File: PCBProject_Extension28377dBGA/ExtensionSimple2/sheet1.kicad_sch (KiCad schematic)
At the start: 86 parts, among them P1 Header 6X2, P2 Header 6X2, P3 Header 2X2, P4 Header 2X2, P5 Header 2X2, P6 Header 2X2, Q1 FMMT618TA, U1 SN74ABT541, U2 SN74ABT541

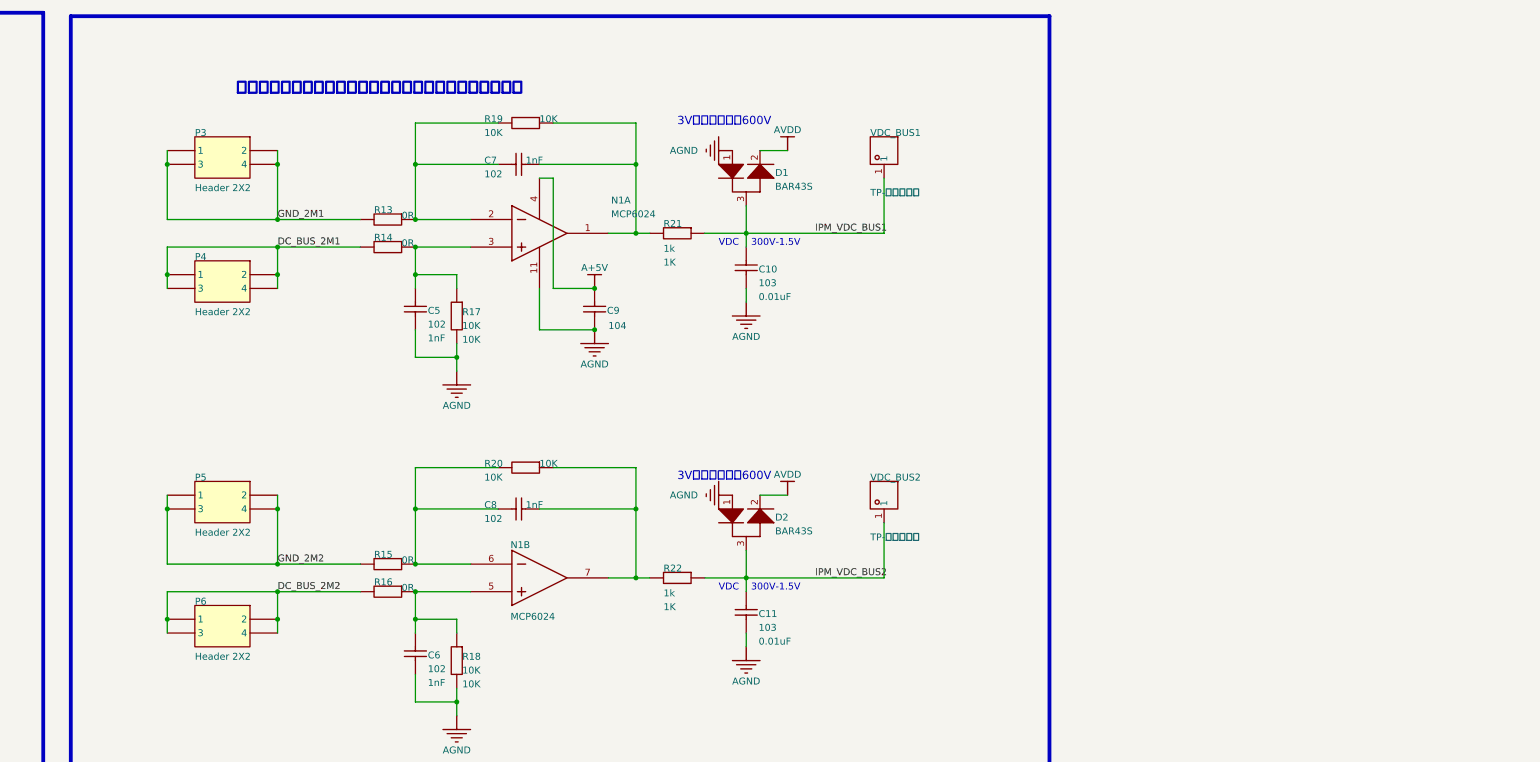
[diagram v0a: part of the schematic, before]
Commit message: block routing done.
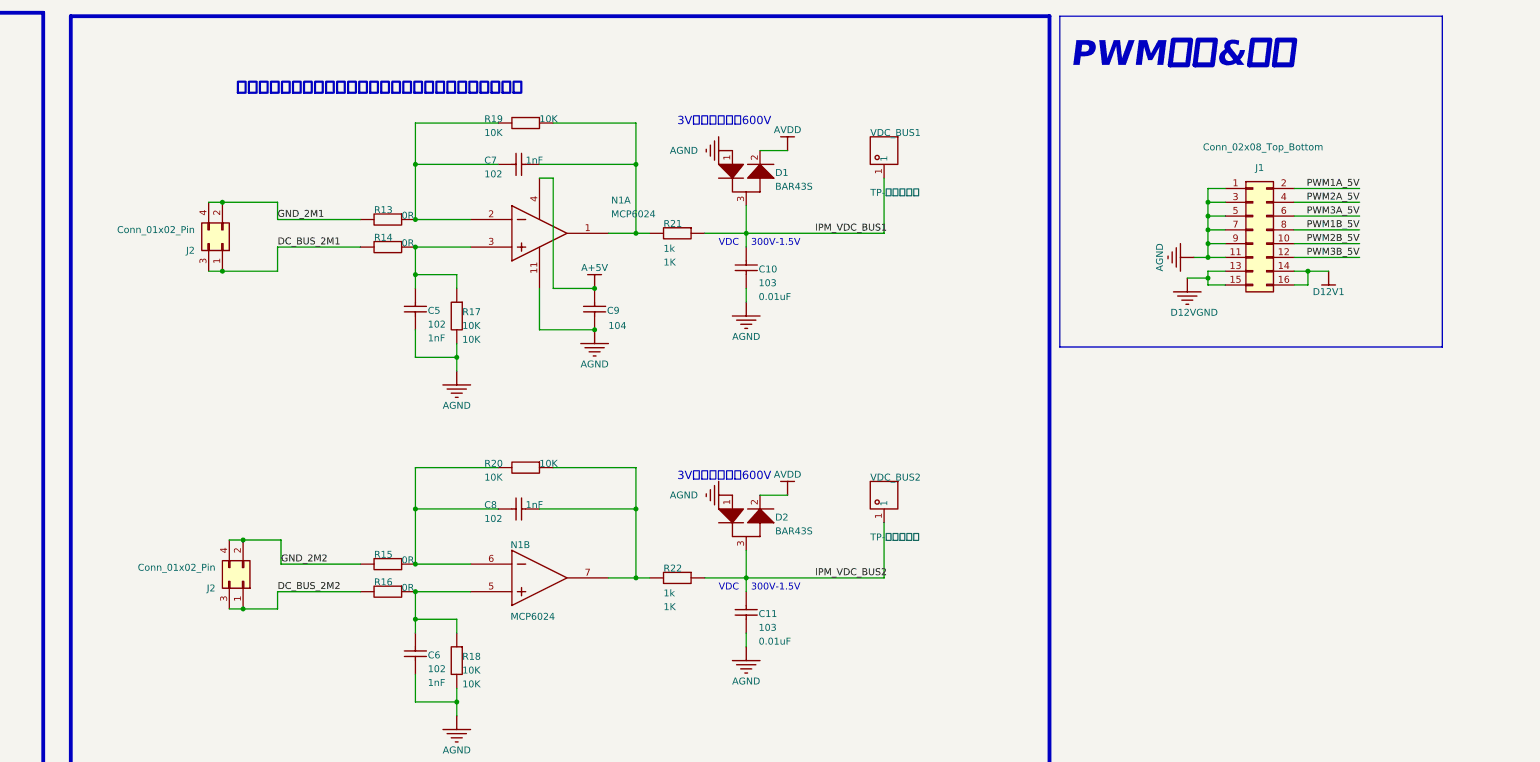
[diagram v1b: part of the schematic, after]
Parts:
- removed P3, P4, P5, P6: Header 2X2, Connector_PinSocket_2.54mm:PinSocket_2x02_P2.54mm_Vertical, symbol sheet1-altium-import:root_0_Header 2X2
- added J1: Conn_02x08_Top_Bottom, Connector_PinSocket_2.54mm:PinSocket_2x08_P2.54mm_Vertical, symbol Connector_Generic:Conn_02x08_Odd_Even
- added J2 (x2): Conn_01x02_Pin, Connector_PinSocket_2.54mm:PinSocket_2x02_P2.54mm_Vertical, symbol Connector_Generic:Conn_02x02_Odd_Even
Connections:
- net AGND: now also J1.1 (Pin_1), J1.11 (Pin_11), J1.3 (Pin_3), J1.5 (Pin_5), J1.7 (Pin_7), J1.9 (Pin_9)
- net D12V1: now also J1.14 (Pin_14), J1.16 (Pin_16)
- net DC_BUS_2M1: now also J2.1 (Pin_1), J2.3 (Pin_3)
- net DC_BUS_2M2: now also J2.1 (Pin_1), J2.3 (Pin_3)
- net GND_2M1: now also J2.2 (Pin_2), J2.4 (Pin_4)
- net GND_2M2: now also J2.2 (Pin_2), J2.4 (Pin_4)
- net PWM1A_5V: now also J1.2 (Pin_2)
- net PWM1B_5V: now also J1.8 (Pin_8)
- net PWM2A_5V: now also J1.4 (Pin_4)
- net PWM2B_5V: now also J1.10 (Pin_10)
- net PWM3A_5V: now also J1.6 (Pin_6)
- net PWM3B_5V: now also J1.12 (Pin_12)
- new net D12VGND: J1.13 (Pin_13), J1.15 (Pin_15)
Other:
- note added: "PWM信号&供电"
